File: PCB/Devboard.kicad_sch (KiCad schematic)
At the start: 0 parts

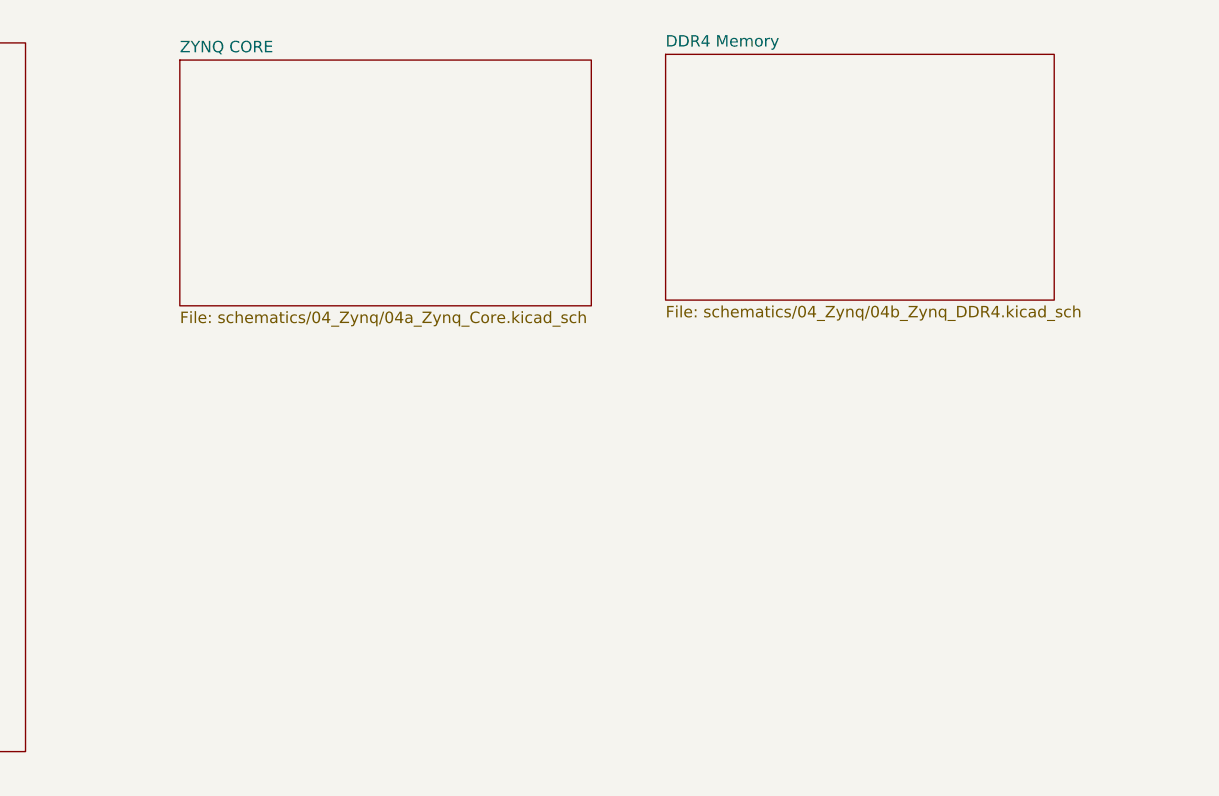
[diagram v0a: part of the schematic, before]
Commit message: Feat: Completed Zynq Core
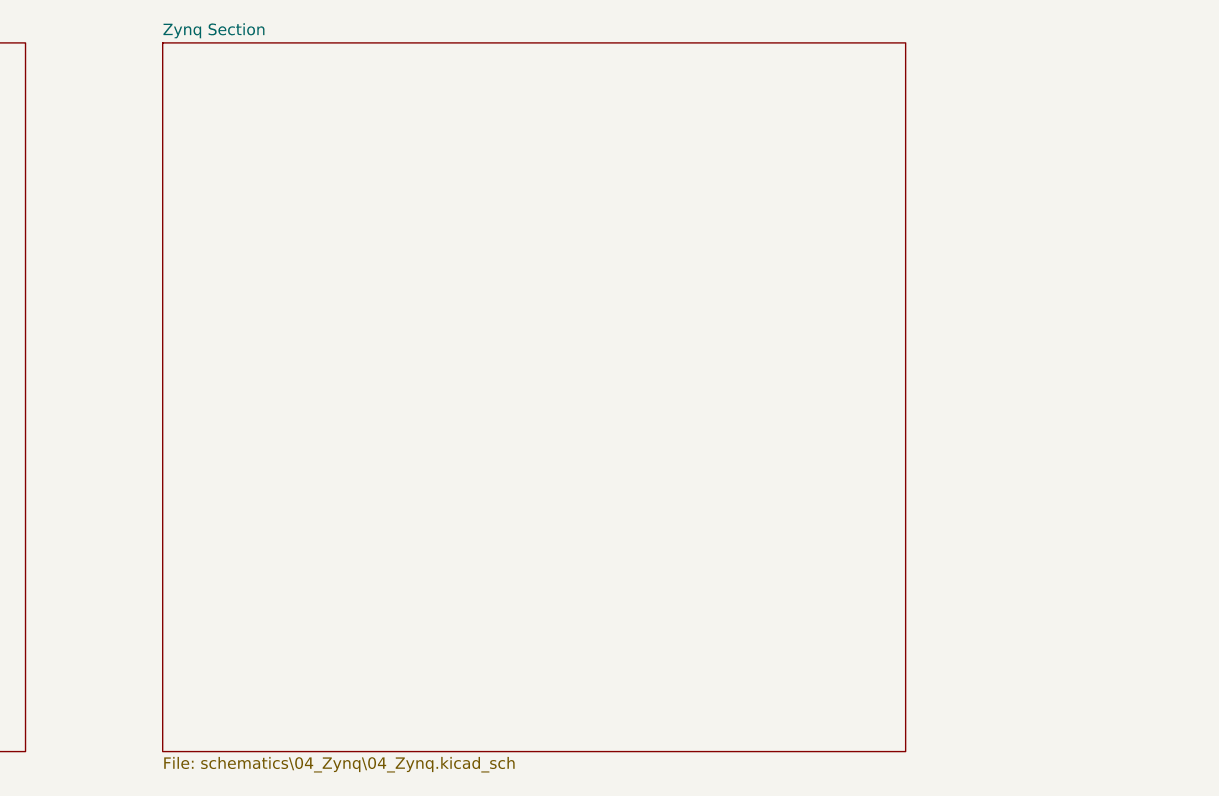
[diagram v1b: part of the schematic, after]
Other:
- removed sheet DDR4 Memory
- removed sheet ZYNQ CORE
- added sheet Zynq Section (schematics\04_Zynq\04_Zynq.kicad_sch)
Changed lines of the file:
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@@
 	(paper "A2")
-	(sheet
-		(at 379.095 15.875)
-		(size 43.18 27.305)
-		(exclude_from_sim no)
-		(in_bom yes)
-		(on_board yes)
-		(dnp no)
-		(fields_autoplaced yes)
-		(stroke
-			(width 0.1524)
-			(type solid)
-		)
-		(fill
-			(color 0 0 0 0)
-		)
-		(property "Sheetname" "DDR4 Memory"
-			(at 379.095 15.1634 0)
-			(show_name no)
-			(do_not_autoplace no)
-			(effects
-				(font
-					(size 1.27 1.27)
-				)
-				(justify left bottom)
-			)
-		)
-		(property "Sheetfile" "schematics/04_Zynq/04b_Zynq_DDR4.kicad_sch"
-			(at 379.095 43.7646 0)
-			(show_name no)
-			(do_not_autoplace no)
-			(effects
-				(font
-					(size 1.27 1.27)
-				)
-				(justify left top)
-			)
-		)
-		(instances
-			(project "Devboard"
-				(path "/f4f7837f-dd80-4f77-b150-4534de1c10d6"
-					(page "6")
-				)
-			)
-		)
-	)
 	(sheet
 		(at 222.885 14.605)
@@
 	)
 	(sheet
-		(at 325.12 16.51)
-		(size 45.72 27.305)
-		(exclude_from_sim no)
-		(in_bom yes)
-		(on_board yes)
-		(dnp no)
-		(fields_autoplaced yes)
-		(stroke
-			(width 0.1524)
-			(type solid)
-		)
-		(fill
-			(color 0 0 0 0)
-		)
-		(property "Sheetname" "ZYNQ CORE"
-			(at 325.12 15.7984 0)
-			(show_name no)
-			(do_not_autoplace no)
-			(effects
-				(font
-					(size 1.27 1.27)
-				)
-				(justify left bottom)
-			)
-		)
-		(property "Sheetfile" "schematics/04_Zynq/04a_Zynq_Core.kicad_sch"
-			(at 325.12 44.3996 0)
-			(show_name no)
-			(do_not_autoplace no)
-			(effects
-				(font
-					(size 1.27 1.27)
-				)
-				(justify left top)
-			)
-		)
-		(instances
-			(project "Devboard"
-				(path "/f4f7837f-dd80-4f77-b150-4534de1c10d6"
-					(page "5")
-				)
-			)
-		)
-	)
-	(sheet
 		(at 15.24 15.24)
 		(size 86.36 78.105)
@@
 				)
 			)
+		)
+	)
+	(sheet
+		(at 323.215 14.605)
+		(size 82.55 78.74)
+		(exclude_from_sim no)
+		(in_bom yes)
+		(on_board yes)
+		(dnp no)
+		(fields_autoplaced yes)
+		(stroke
+			(width 0.1524)
+			(type solid)
+		)
+		(fill
+			(color 0 0 0 0)
+		)
+		(property "Sheetname" "Zynq Section"
+			(at 323.215 13.8934 0)
+			(show_name no)
+			(do_not_autoplace no)
+			(effects
+				(font
+					(size 1.27 1.27)
+				)
+				(justify left bottom)
+			)
+		)
+		(property "Sheetfile" "schematics\\04_Zynq\\04_Zynq.kicad_sch"
+			(at 323.215 93.9296 0)
+			(show_name no)
+			(do_not_autoplace no)
+			(effects
+				(font
+					(size 1.27 1.27)
+				)
+				(justify left top)
+			)
+		)
+		(instances
+			(project "Devboard"
+				(path "/f4f7837f-dd80-4f77-b150-4534de1c10d6"
+					(page "5")
+				)
+			)
